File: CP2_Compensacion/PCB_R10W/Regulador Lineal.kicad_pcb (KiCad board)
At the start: 2 copper layers, 64 x 51 mm, 27 parts, among them J1 I1, J2 I2, J3 I3, J4 gnd, J5 out, J6 V1, J7 in, Q1 BD140, Q10 BD139, Q2 BD140, Q3 BD139, Q4 BD139, Q5 TIP42C, Q6 BD139, Q7 BD139, Q8 BD139, U1 TL431LP

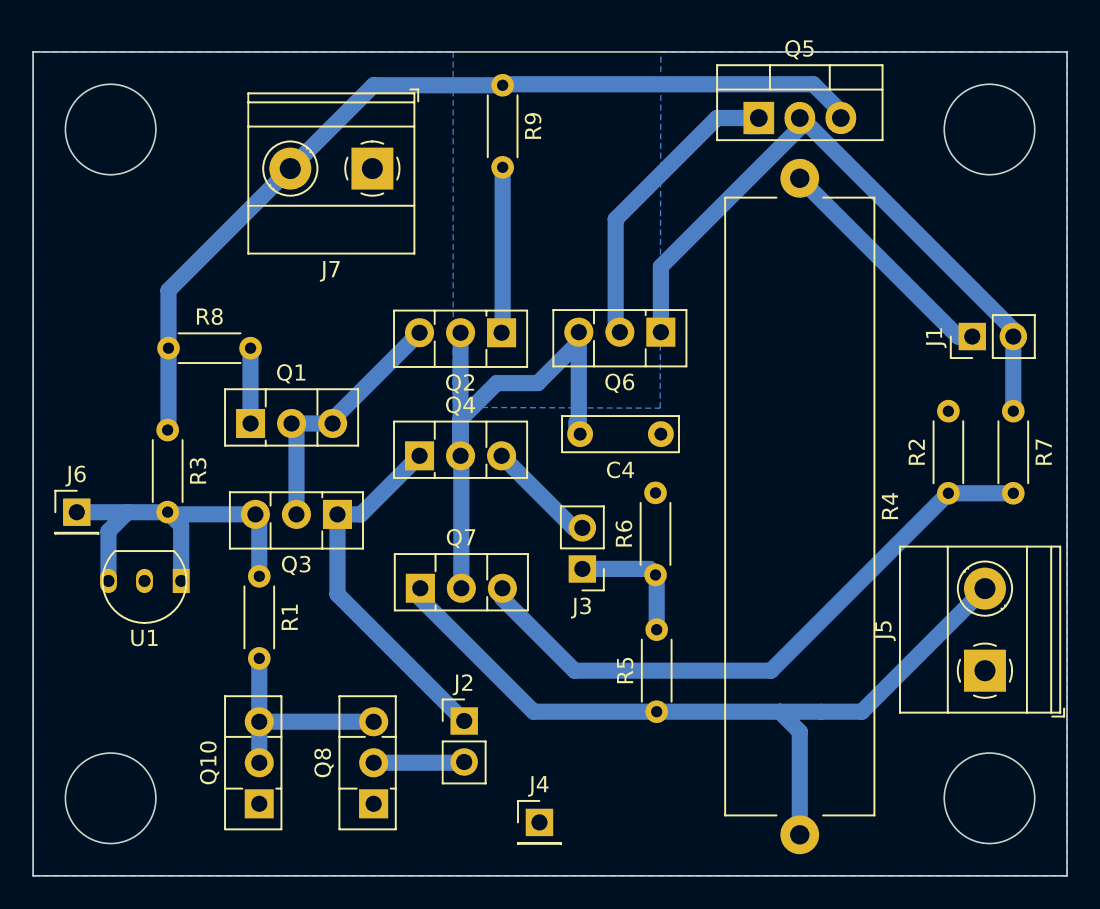
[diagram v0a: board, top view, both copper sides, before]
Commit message: Archivos de Fabricacion
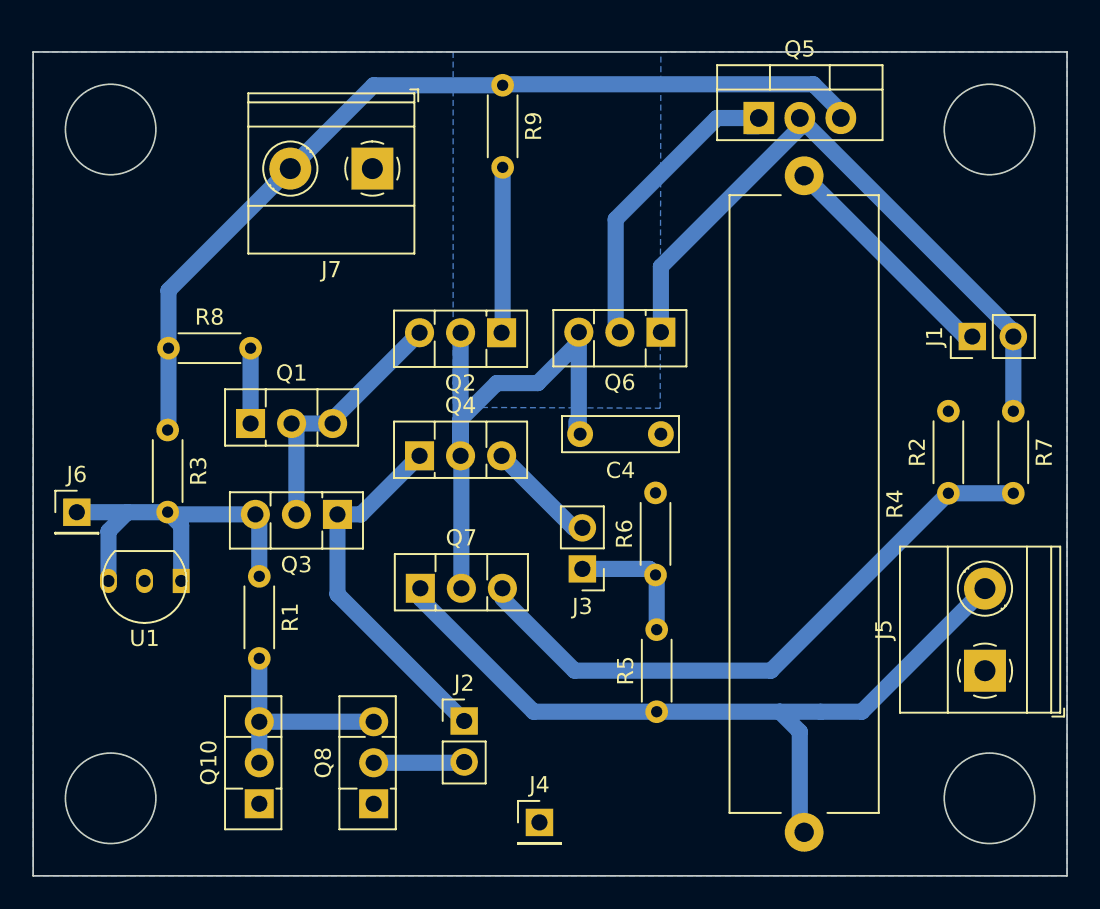
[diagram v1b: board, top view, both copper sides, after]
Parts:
- moved R4 0.31 mm to (242.8, 50.6)
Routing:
- net Net-(Q7-B): track 38.7 -> 38.0 mm
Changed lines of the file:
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@@
 		(tenting front back)
 		(pcbplotparams
-			(layerselection 0x00000000_00000000_55555555_5755f5ff)
+			(layerselection 0x00000000_00000000_55555555_57555555)
 			(plot_on_all_layers_selection 0x00000000_00000000_00000000_00000000)
 			(disableapertmacros no)
@@
 			(outputformat 1)
 			(mirror no)
-			(drillshape 1)
+			(drillshape 0)
 			(scaleselection 1)
-			(outputdirectory "")
+			(outputdirectory "Salida/")
 		)
 	)
@@
 	(footprint "Resistor_THT:R_Axial_Power_L38.0mm_W9.0mm_P40.64mm"
 		(layer "F.Cu")
-		(at 242.536485 50.8 -90)
+		(at 242.807184 50.644095 -90)
 		(descr "Resistor, Axial_Power series, Box, pin pitch=40.64mm, 9W, length*width*height=38*9*9mm^3, http://cdn-reichelt.de/documents/datenblatt/B400/5WAXIAL_9WAXIAL_11WAXIAL_17WAXIAL%23YAG.pdf")
 		(tags "Resistor Axial_Power series Box pin pitch 40.64mm 9W length 38mm width 9mm height 9mm")
@@
 	)
 	(segment
-		(start 252.333573 60.597088)
-		(end 242.536485 50.8)
+		(start 253.215157 60.597088)
+		(end 252.760177 60.597088)
 		(width 1)
 		(layer "B.Cu")
@@
 	)
 	(segment
-		(start 253.215157 60.597088)
-		(end 252.333573 60.597088)
+		(start 252.760177 60.597088)
+		(end 242.807184 50.644095)
 		(width 1)
 		(layer "B.Cu")
@@
 	)
 	(segment
-		(start 224.128641 76.808641)
-		(end 224.128641 76.18)
-		(width 1)
-		(layer "B.Cu")
-		(net 8)
-	)
-	(segment
 		(start 240.753544 81.28)
 		(end 228.6 81.28)
@@
 	)
 	(segment
-		(start 226.32 63.48)
-		(end 228.86 60.94)
+		(start 221.588641 76.18)
+		(end 221.588641 68.028641)
 		(width 1)
 		(layer "B.Cu")
@@
 	(segment
 		(start 221.588641 68.028641)
-		(end 221.588641 76.18)
+		(end 221.54 67.98)
+		(width 1)
+		(layer "B.Cu")
+		(net 11)
+	)
+	(segment
+		(start 226.32 63.48)
+		(end 228.86 60.94)
 		(width 1)
 		(layer "B.Cu")
@@
 	)
 	(segment
-		(start 221.54 67.98)
-		(end 221.588641 68.028641)
-		(width 1)
-		(layer "B.Cu")
-		(net 11)
-	)
-	(segment
 		(start 221.54 65.72)
 		(end 223.78 63.48)
@@
 	)
 	(segment
-		(start 255.755157 65.217663)
-		(end 255.755157 60.597088)
+		(start 255.755157 60.597088)
+		(end 255.755157 60.28439)
 		(width 1)
 		(layer "B.Cu")
@@
 	)
 	(segment
-		(start 242.54 47.668805)
-		(end 233.94 56.268805)
+		(start 255.755157 65.217663)
+		(end 255.755157 60.597088)
 		(width 1)
 		(layer "B.Cu")
@@
 	)
 	(segment
-		(start 255.755157 60.175157)
-		(end 242.649233 47.069233)
+		(start 242.54 47.668805)
+		(end 233.94 56.268805)
 		(width 1)
 		(layer "B.Cu")
@@
 		(width 1)
 		(layer "B.Cu")
+		(net 17)
+	)
+	(segment
+		(start 255.755157 60.28439)
+		(end 242.54 47.069233)
+		(width 1)
+		(layer "B.Cu")
